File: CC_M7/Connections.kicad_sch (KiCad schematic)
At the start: 12 parts, among them J1 Conn_01x04_Pin, J10 Conn_01x04_Pin, J11 USB_B_Micro, J12 Conn_01x04_Pin, J3 Conn_01x03_Pin, J4 Conn_01x03_Pin, J5 Conn_01x03_Pin, J6 Conn_01x03_Pin, J7 Conn_01x03_Pin, J8 Conn_01x03_Pin

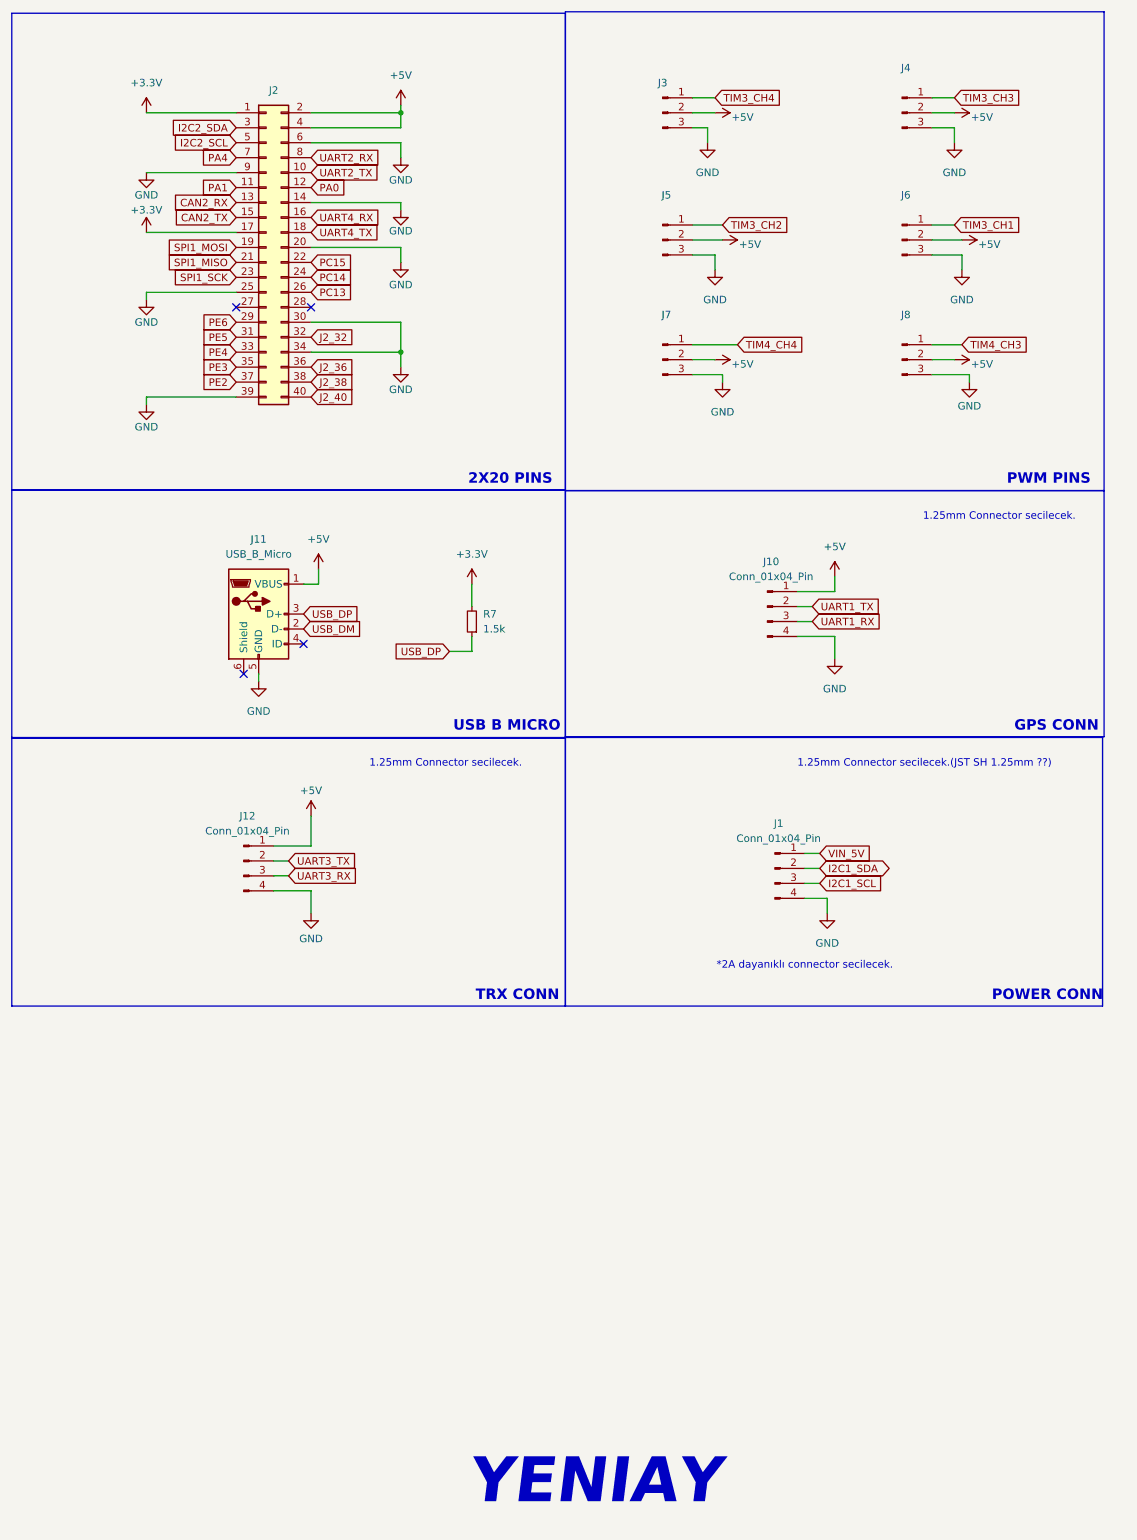
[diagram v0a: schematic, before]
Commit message: last control
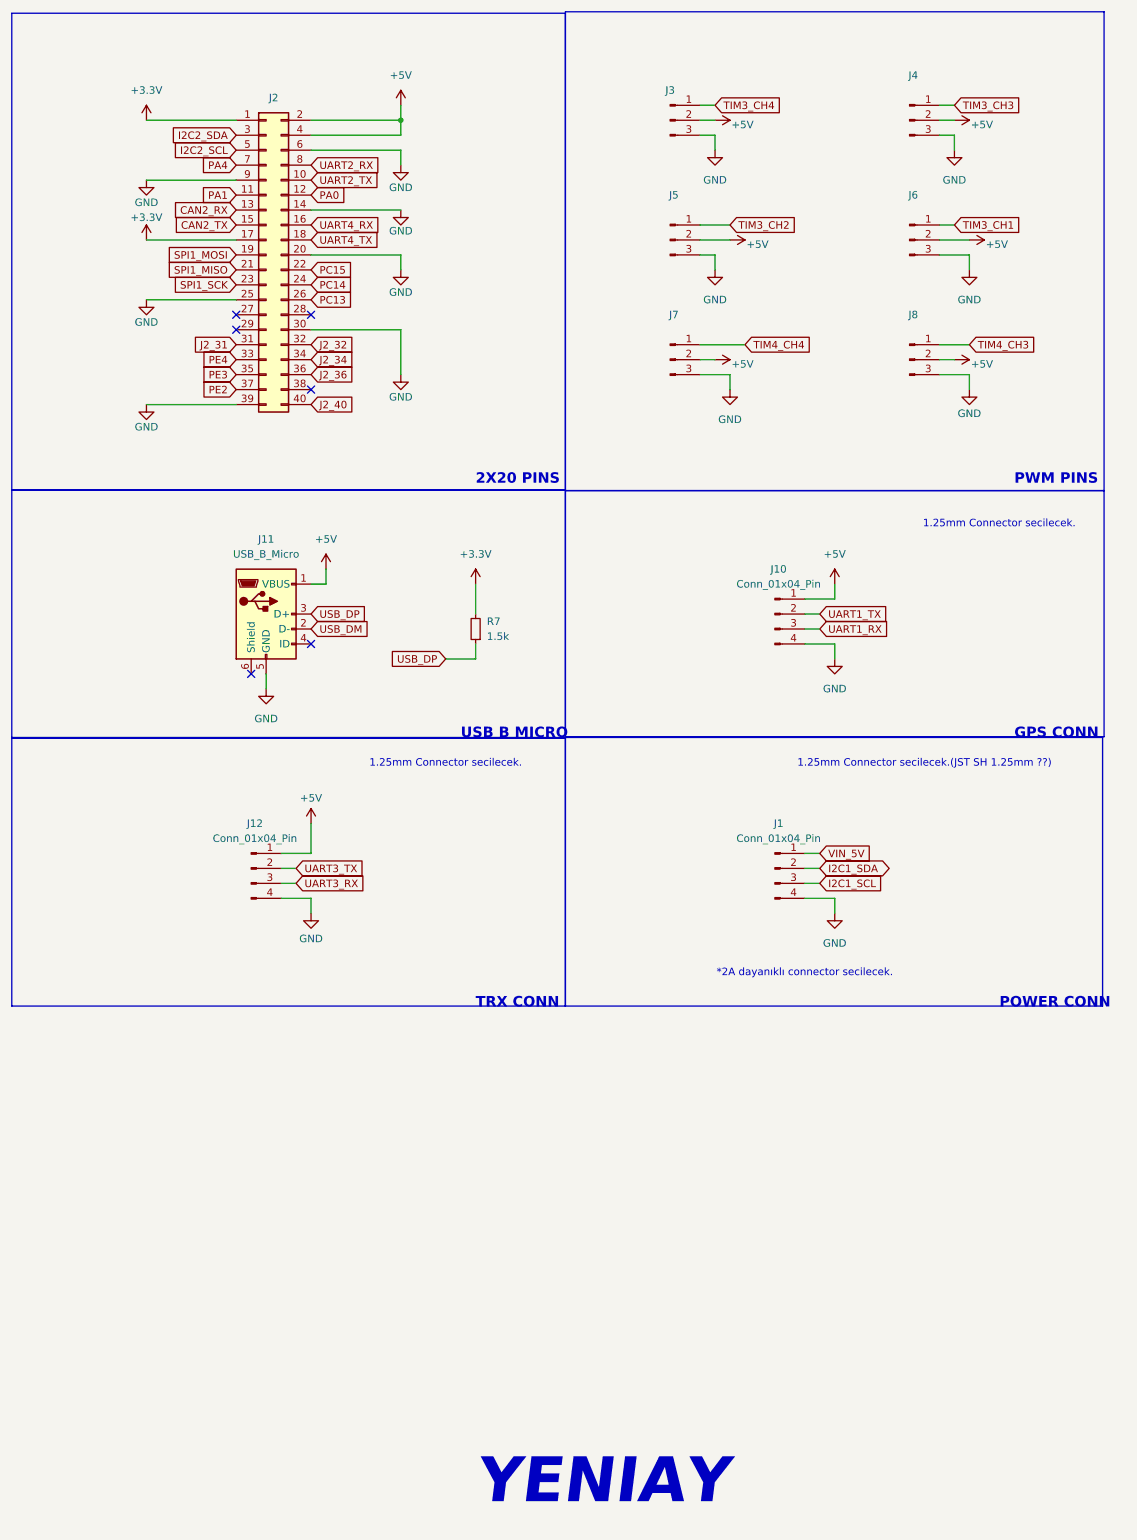
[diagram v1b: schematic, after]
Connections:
- net GND: no longer J2.34 (Pin_34)
- net J2_38: no longer names the net of J2.38 (Pin_38)
- net PE5 renamed J2_31
- net PE6: no longer names the net of J2.29 (Pin_29)
- new net J2_34: J2.34 (Pin_34)
- no-connect marks 4 -> 6
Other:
- moved on the sheet: J10, J11, J12, J2, J3, J4, J5, J6, J7, J8, R7
